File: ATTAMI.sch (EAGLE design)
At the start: 27 parts, among them Q1 NTD3055L, Q2 NTD3055L, Q3 NTD3055L, SW1 SPST_TACT-KMR2, U1 NCP4626 (5V), U2 ATTINY85

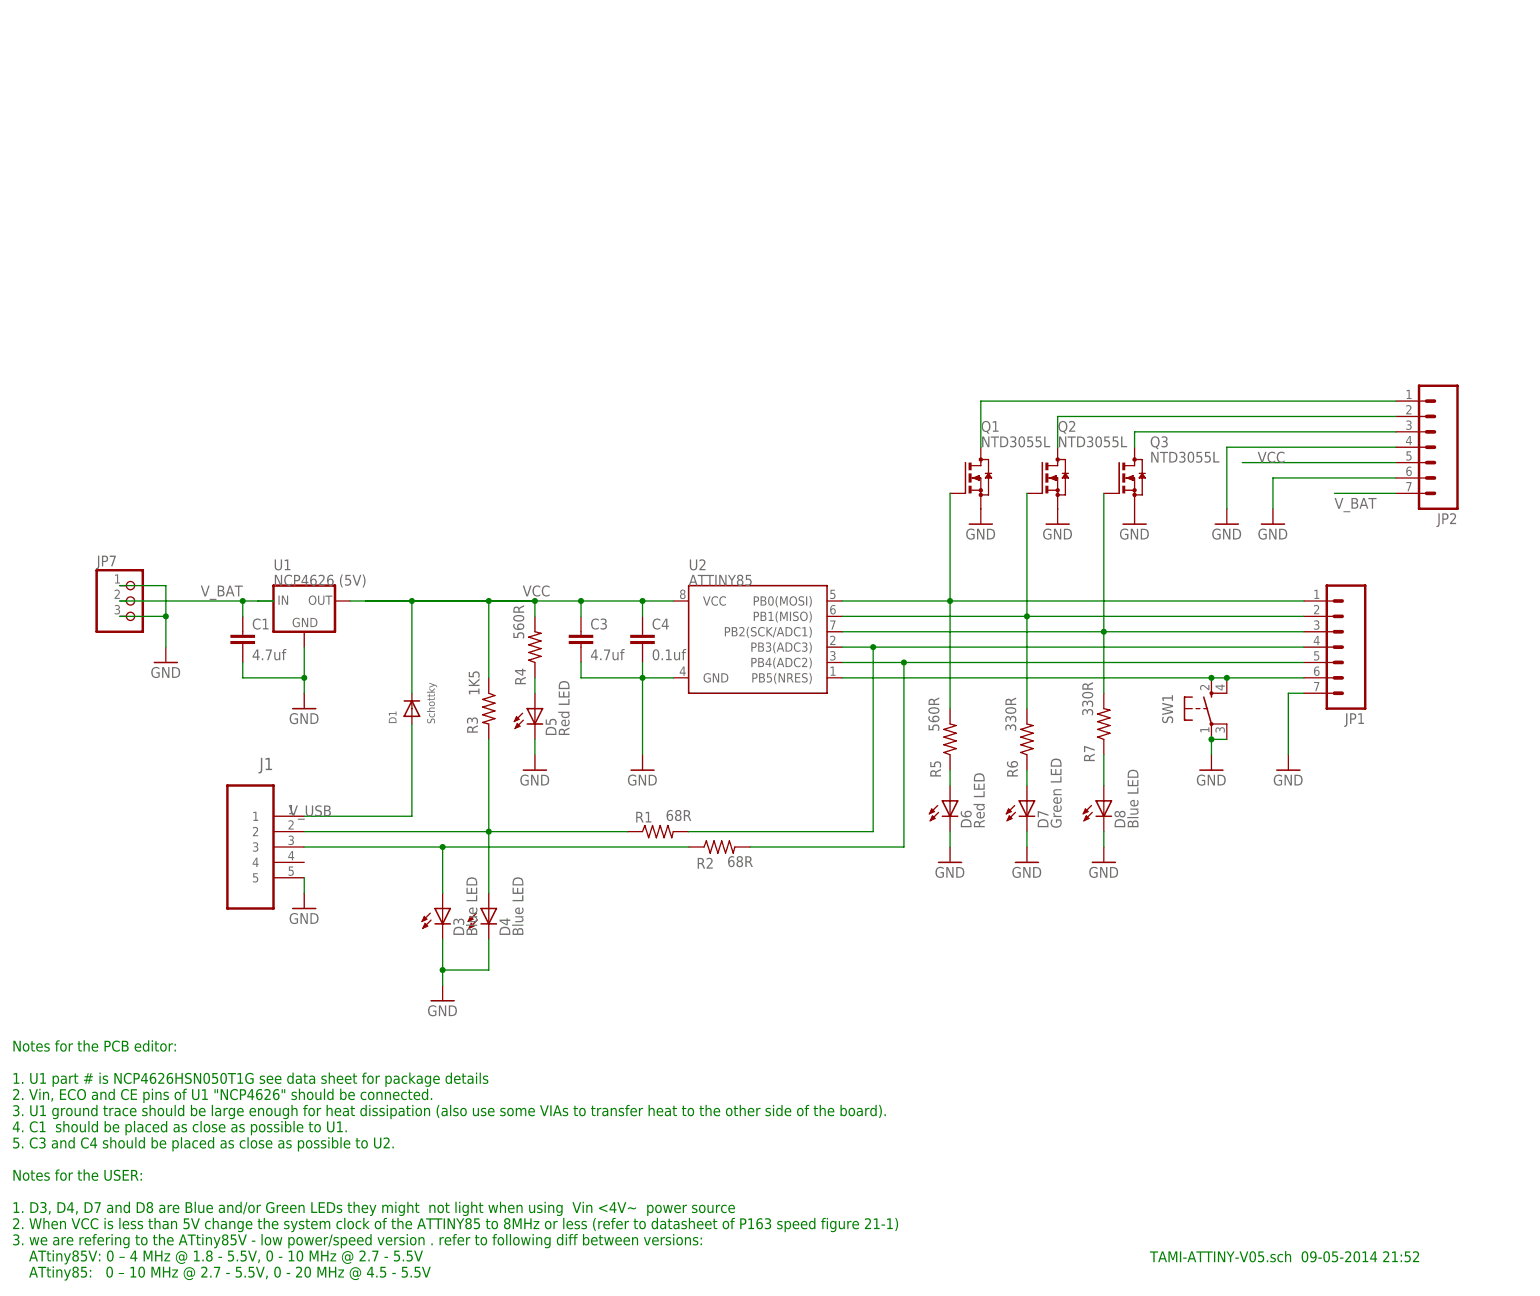
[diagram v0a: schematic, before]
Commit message: ver07
https://dl.dropboxusercontent.com/u/6430706/ShareX/2014/05/TAMI-ATTINY-V07.pdf
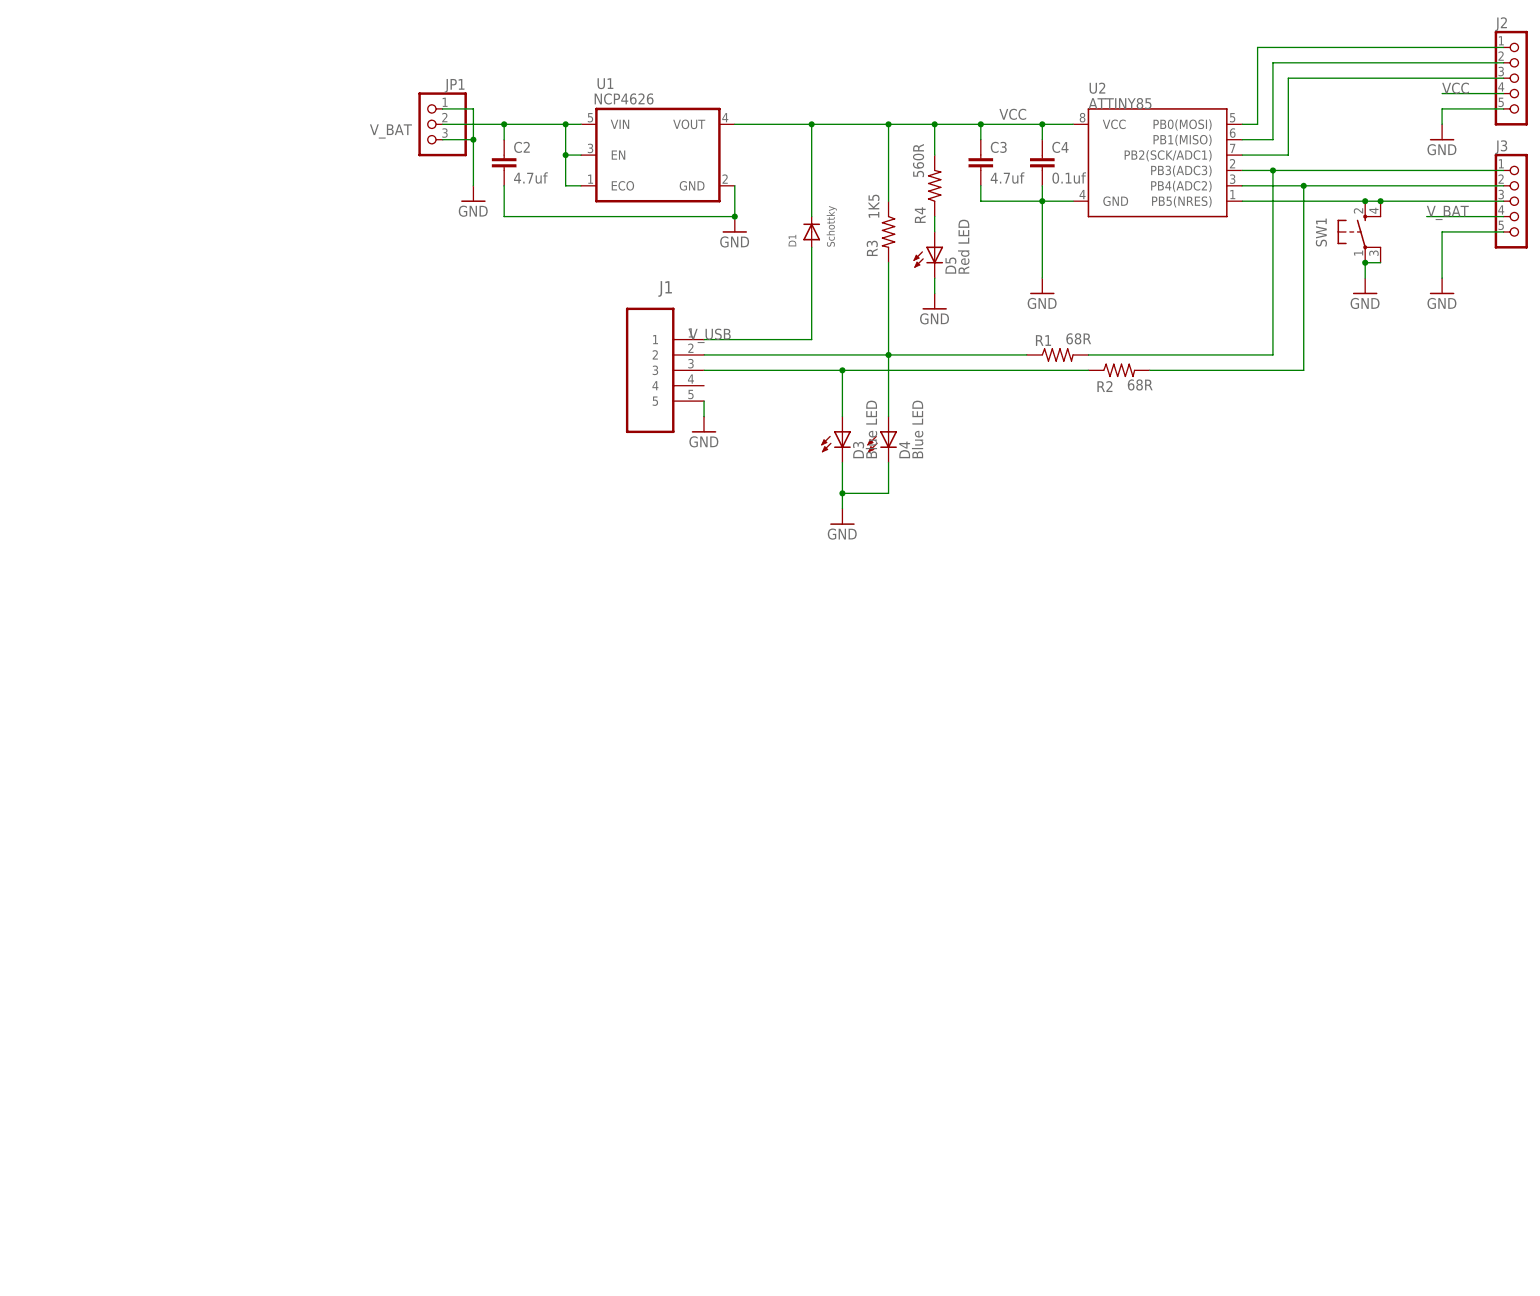
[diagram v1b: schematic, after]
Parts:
- removed C1: 4.7uf, SparkFun:CAP0805
- removed D6: Red LED, SparkFun:LED0603
- removed D7: Green LED, SparkFun:LED0603
- removed D8: Blue LED, SparkFun:LED0603
- removed JP2: (no value), SparkFun:M07
- removed JP7: (no value), microbuilder:HEADER-1X376MIL
- removed Q1, Q2, Q3: NTD3055L, transistor-small-signal:BSS123
- removed R5: 560R, SparkFun:RESISTOR0402-RES
- removed R6, R7: 330R, SparkFun:RESISTOR0402-RES
- added C2: 4.7uf, SparkFun:CAP0805
- added J2, J3: CON_HEADER_1X05-PTH, dp_devices:CON_HEADER_1X05-PTH
- C4: device SparkFun:CAP0402-CAP -> SparkFun:CAP0805
- D1: device microbuilder:DIODESMA -> microbuilder:DIODESOD-323
- D3, D4, D5: device SparkFun:LED0603 -> dp_devices:LED-0805
- JP1: device SparkFun:M07 -> microbuilder:HEADER-1X376MIL
- R1, R2, R3, R4: device SparkFun:RESISTOR0402-RES -> SparkFun:RESISTOR0805-RES
- U1: value NCP4626 (5V) -> NCP4626; device v-reg:LP2950CDT-3.0 -> yair_r:NCP4626
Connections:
- removed net N$12: D7.A, R6.1
- removed net N$13: D6.A, R5.1
- removed net N$14: D8.A, R7.1
- removed net N$16: JP2.3, Q3.D
- removed net N$4: JP2.2, Q2.D
- removed net N$9: JP2.1, Q1.D
- net GND: now also C2.2, J2.5, J3.5, JP1.1, JP1.3; no longer C1.2, D6.C, D7.C, D8.C, JP1.7, JP2.4, JP2.6, JP7.1, JP7.3, Q1.S, Q2.S, Q3.S
- net N$1: now also J3.1; no longer JP1.4
- net N$15: now also J2.2; no longer JP1.2, Q2.G, R6.2
- net N$3: now also J2.1; no longer JP1.1, Q1.G, R5.2
- net N$5: now also J2.3; no longer JP1.3, Q3.G, R7.2
- net N$6: now also J3.2; no longer JP1.5
- net N$8: now also J3.3; no longer JP1.6
- net VCC: now also J2.4, U1.VOUT; no longer JP2.5, U1.OUT
- net V_BAT: now also C2.1, J3.4, JP1.2, U1.ECO, U1.EN, U1.VIN; no longer C1.1, JP7.2, U1.IN
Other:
- note added: "Notes for the PCB editor: 1. U1 ground trace should be large enough for heat dissipation (also use some VIAs to transfer heat to the other side of the board). 2. C1 should be placed as close as possible to U1. 3. C3 and C4 should be placed as close as possible to U2. Notes for the USER: 1. D3, D4 and D5 are Blue and/or Green LEDs they might not light when using Vin <4V~ power source 2. When VCC i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"
- note added: "T.A.M.I hackerspace crew LICENSE: CERN OHL 1.7"
- note removed: "Notes for the PCB editor: 1. U1 part # is NCP4626HSN050T1G see data sheet for package details 2. Vin, ECO and CE pins of U1 "NCP4626" should be connected. 3. U1 ground trace should be large enough for heat dissipation (also use some VIAs to transfer heat to the other side of the board). 4. C1 should be placed as close as possible to U1. 5. C3 and C4 should be placed as close as possible to U2. No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"
- note removed: "TAMI-ATTINY-V05.sch 09-05-2014 21:52"
- moved on the sheet: C3, C4, D1, J1, R1, R2, R3, R4, SW1, U2
